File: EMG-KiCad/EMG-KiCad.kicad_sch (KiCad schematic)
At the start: 11 parts, among them U1 AD623, U2 OPA1662D, U3 OPA1662D

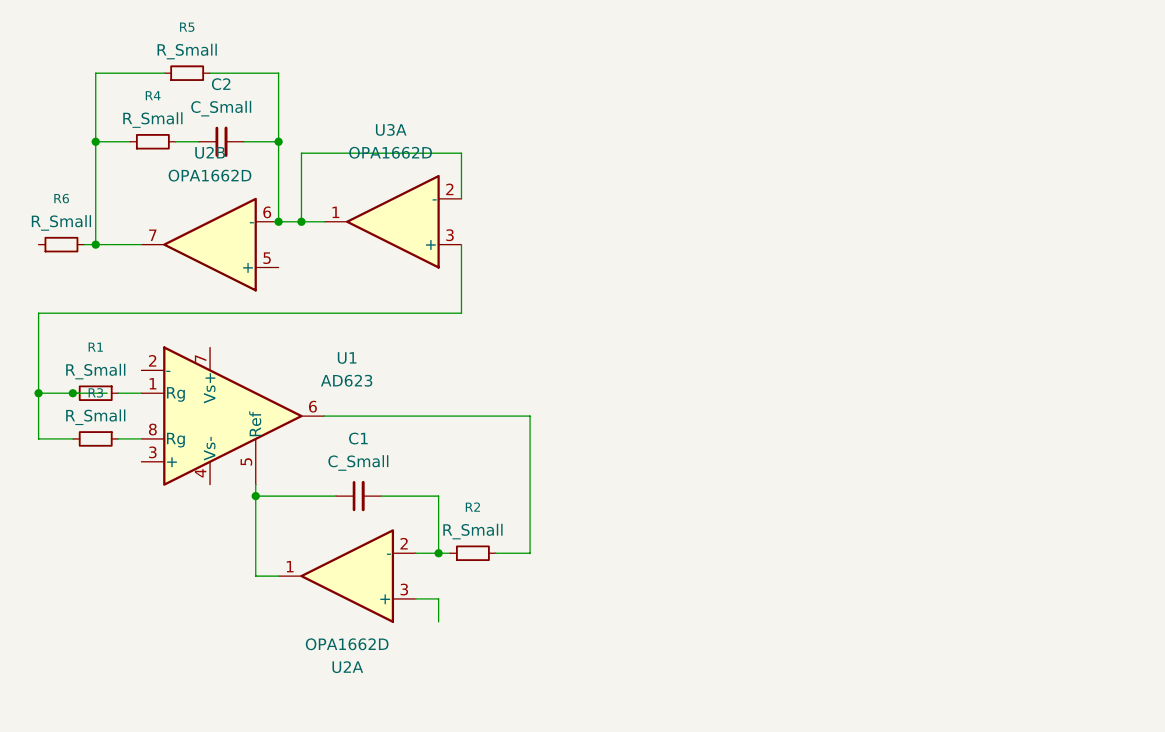
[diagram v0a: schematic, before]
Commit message: Amplifiedx2
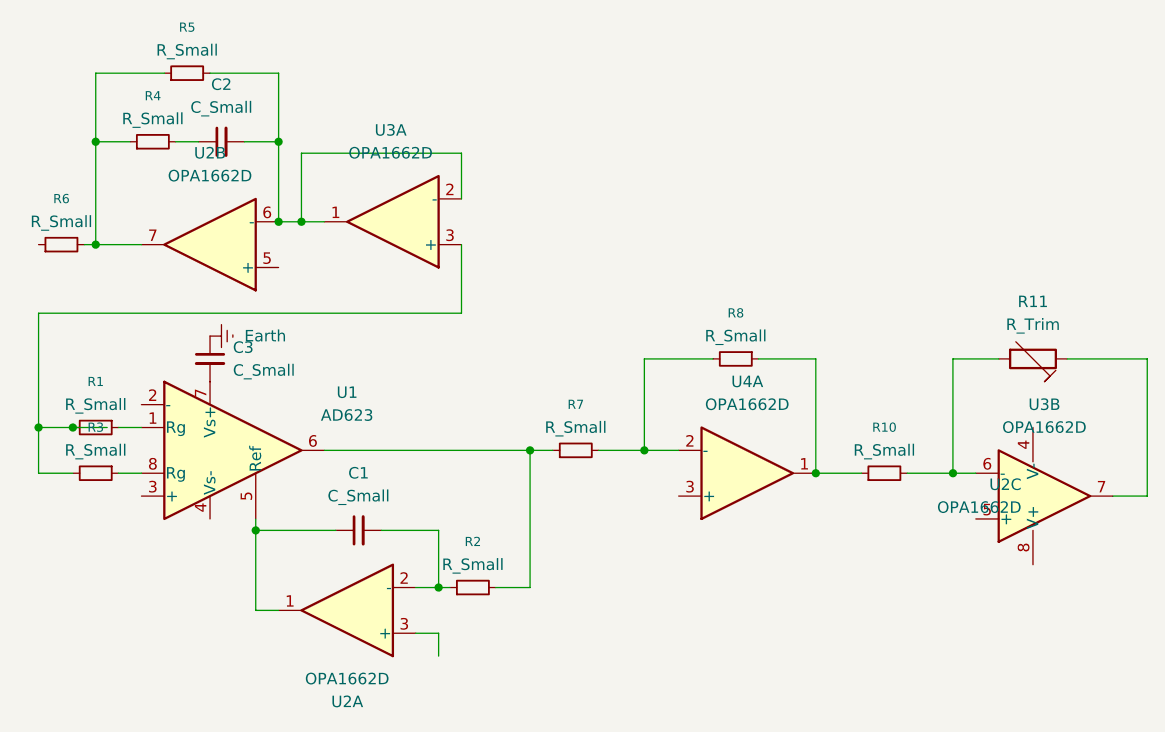
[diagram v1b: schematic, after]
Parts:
- added C3: C_Small, symbol Device:C_Small
- added R10, R7, R8: R_Small, symbol Device:R_Small
- added R11: R_Trim, symbol Device:R_Trim
- added unit 3 of U2
- added unit 2 of U3
- added U4: OPA1662D, Package_SO:SOIC-8_3.9x4.9mm_P1.27mm, symbol Amplifier_Operational:OPA1662D
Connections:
- net at R2.2, U1.6: now also R7.1
- net at U1.7 (Vs+): now also C3.2
- new net: R7.2, R8.2, U4.2 (-)
- new net: R10.1, R8.1, U4.1
- new net: R11.1, U3.7
- new net: R10.2, R11.2, U3.6 (-)
- new net Earth: C3.1
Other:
- moved on the sheet: C1, R1, R2, R3, U1, U2A
